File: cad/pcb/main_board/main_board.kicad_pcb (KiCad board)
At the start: 2 copper layers, 70.5 x 56.5 mm, 76 parts, among them J1 USB_B_Micro, J2 Conn_ARM_JTAG_SWD_10, U1 STM32F401R_B-C_Tx, U2 TLV75533PDRVR, Y1 Crystal_GND23

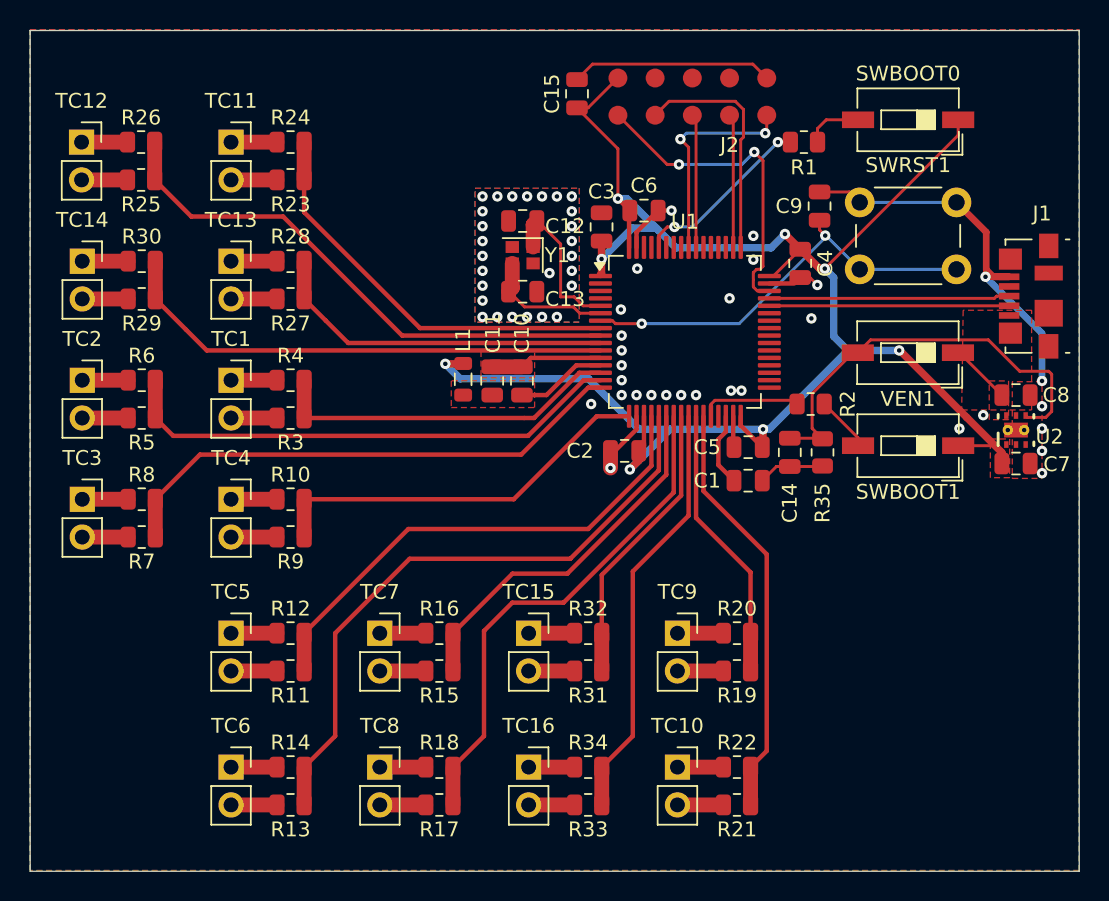
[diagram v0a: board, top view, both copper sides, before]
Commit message: Update main_board.kicad_pcb
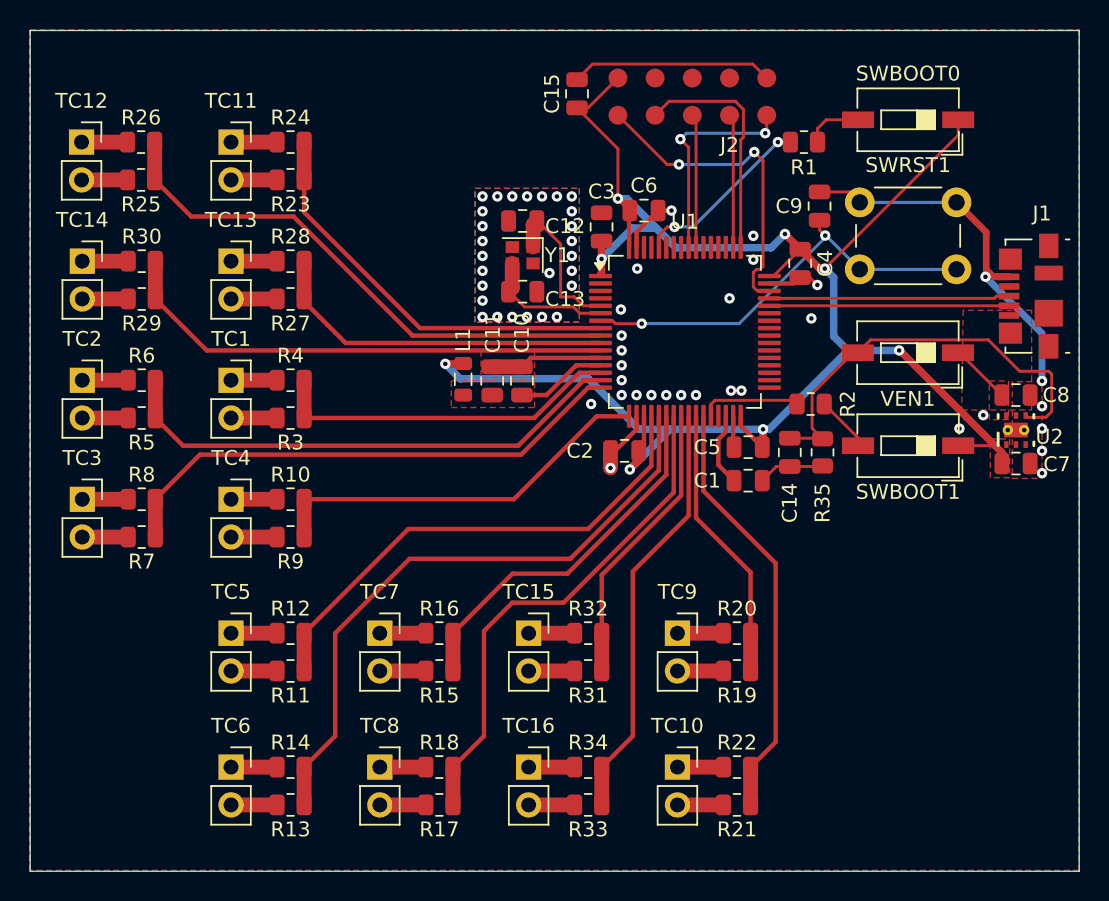
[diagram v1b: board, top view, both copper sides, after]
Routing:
- net /MCU/ADC_IN1: track 34.5 -> 35.0 mm
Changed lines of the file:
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@@
+	)
+	(segment
+		(start 102.7 56)
+		(end 98.3 60.4)
+		(width 0.3)
+		(layer "F.Cu")
+		(net 20)
 	)
 	(segment
@@
 	)
 	(segment
-		(start 98.96 59.74)
-		(end 75.1125 59.74)
+		(start 98.3 60.4)
+		(end 75.7725 60.4)
 		(width 0.3)
 		(layer "F.Cu")
@@
 	)
 	(segment
-		(start 75.1125 59.74)
+		(start 75.7725 60.4)
 		(end 73.9125 58.54)
-		(width 0.3)
-		(layer "F.Cu")
-		(net 20)
-	)
-	(segment
-		(start 102.7 56)
-		(end 98.96 59.74)
 		(width 0.3)
 		(layer "F.Cu")
@@
 	)
 	(segment
+		(start 115.6 80.3125)
+		(end 113.9125 82)
+		(width 0.3)
+		(layer "F.Cu")
+		(net 36)
+	)
+	(segment
 		(start 110.75 63.45)
-		(end 115 67.7)
+		(end 115.6 68.3)
+		(width 0.3)
+		(layer "F.Cu")
+		(net 36)
+	)
+	(segment
+		(start 113.9125 84.54)
+		(end 113.9125 82)
+		(width 1)
+		(layer "F.Cu")
+		(net 36)
+	)
+	(segment
+		(start 115.6 68.3)
+		(end 115.6 80.3125)
 		(width 0.3)
 		(layer "F.Cu")
@@
 	)
 	(segment
-		(start 115 67.7)
-		(end 115 80.9125)
-		(width 0.3)
-		(layer "F.Cu")
-		(net 36)
-	)
-	(segment
-		(start 115 80.9125)
-		(end 113.9125 82)
-		(width 0.3)
-		(layer "F.Cu")
-		(net 36)
-	)
-	(segment
-		(start 113.9125 84.54)
-		(end 113.9125 82)
-		(width 1)
-		(layer "F.Cu")
-		(net 36)
-	)
-	(segment
 		(start 112.0875 82)
 		(end 109 82)
@@
 	)
 	(segment
+		(start 91.2 53)
+		(end 83.2 45)
+		(width 0.3)
+		(layer "F.Cu")
+		(net 40)
+	)
+	(segment
+		(start 103.825 53)
+		(end 91.2 53)
+		(width 0.3)
+		(layer "F.Cu")
+		(net 40)
+	)
+	(segment
+		(start 73.86875 42.54)
+		(end 73.86875 40)
+		(width 1)
+		(layer "F.Cu")
+		(net 40)
+	)
+	(segment
+		(start 83.2 45)
+		(end 76.32875 45)
+		(width 0.3)
+		(layer "F.Cu")
+		(net 40)
+	)
+	(segment
 		(start 76.32875 45)
 		(end 73.86875 42.54)
@@
 	)
 	(segment
-		(start 103.825 53)
-		(end 90.5 53)
-		(width 0.3)
-		(layer "F.Cu")
-		(net 40)
-	)
-	(segment
-		(start 73.86875 42.54)
-		(end 73.86875 40)
-		(width 1)
-		(layer "F.Cu")
-		(net 40)
-	)
-	(segment
-		(start 90.5 53)
-		(end 82.5 45)
-		(width 0.3)
-		(layer "F.Cu")
-		(net 40)
-	)
-	(segment
-		(start 82.5 45)
-		(end 76.32875 45)
-		(width 0.3)
-		(layer "F.Cu")
-		(net 40)
-	)
-	(segment
 		(start 72.04375 40)
 		(end 68.95625 40)
@@
 	)
 	(segment
-		(start 85.3725 52)
+		(start 83.9125 50.7125)
 		(end 83.9125 50.54)
 		(width 0.3)
@@
 	(segment
 		(start 103.825 53.5)
-		(end 86.8725 53.5)
+		(end 86.7 53.5)
 		(width 0.3)
 		(layer "F.Cu")
@@
 	)
 	(segment
-		(start 86.8725 53.5)
-		(end 85.3725 52)
-		(width 0.3)
-		(layer "F.Cu")
+		(start 86.7 53.5)
+		(end 83.9125 50.7125)
+		(width 0.3)
+		(layer "F.Cu")
